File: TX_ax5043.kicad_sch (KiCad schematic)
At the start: 27 parts, among them P6 CONUFL001-SMD-T, P7 CONUFL001-SMD-T, Q7 DMP2037U-7, U23 AX5043

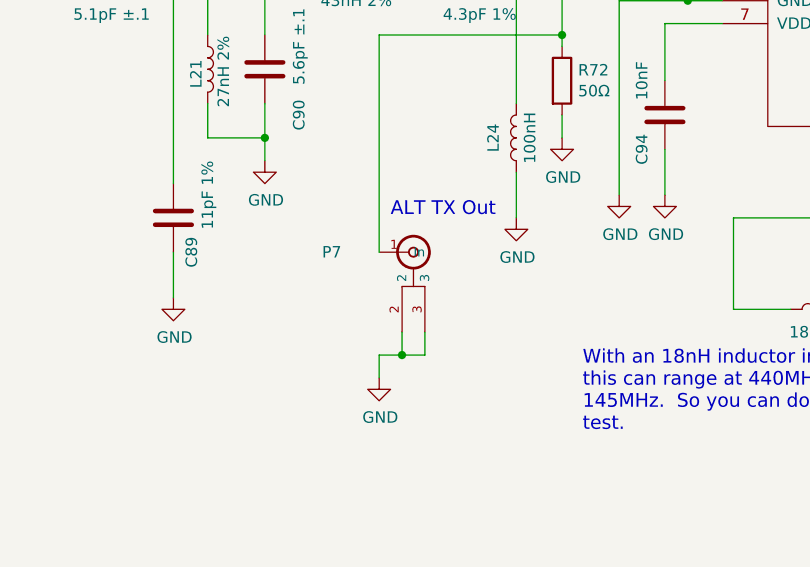
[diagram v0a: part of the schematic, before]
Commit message: More minor tweaks and cleanups
Signed-off-by: Corey Minyard <corey@minyard.net>
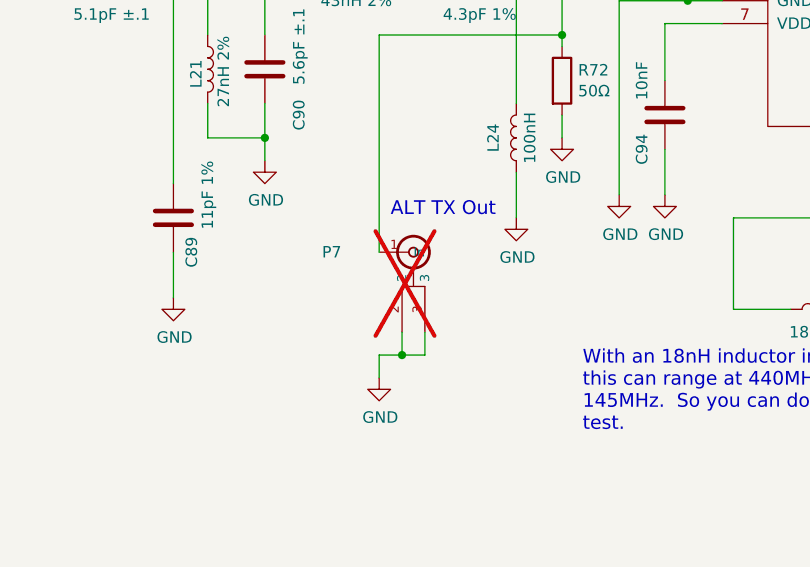
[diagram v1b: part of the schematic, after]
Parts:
- P7: now not fitted; now left out of the parts list
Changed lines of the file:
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@@
 		(unit 1)
 		(exclude_from_sim no)
-		(in_bom yes)
+		(in_bom no)
 		(on_board yes)
-		(dnp no)
+		(dnp yes)
 		(property "Reference" "P7"
 			(at 196.85 170.18 0)
